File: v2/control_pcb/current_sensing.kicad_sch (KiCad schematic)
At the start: 20 parts, among them J14 Conn_02x02_Top_Bottom, J15 Conn_02x02_Top_Bottom, U10 TMCS1108A3UQDR, U11 TMCS1108A3UQDR, U6 TMCS1108A3UQDR, U7 TMCS1108A3UQDR, U8 ADS7828, U9 LM4040LP-4.1

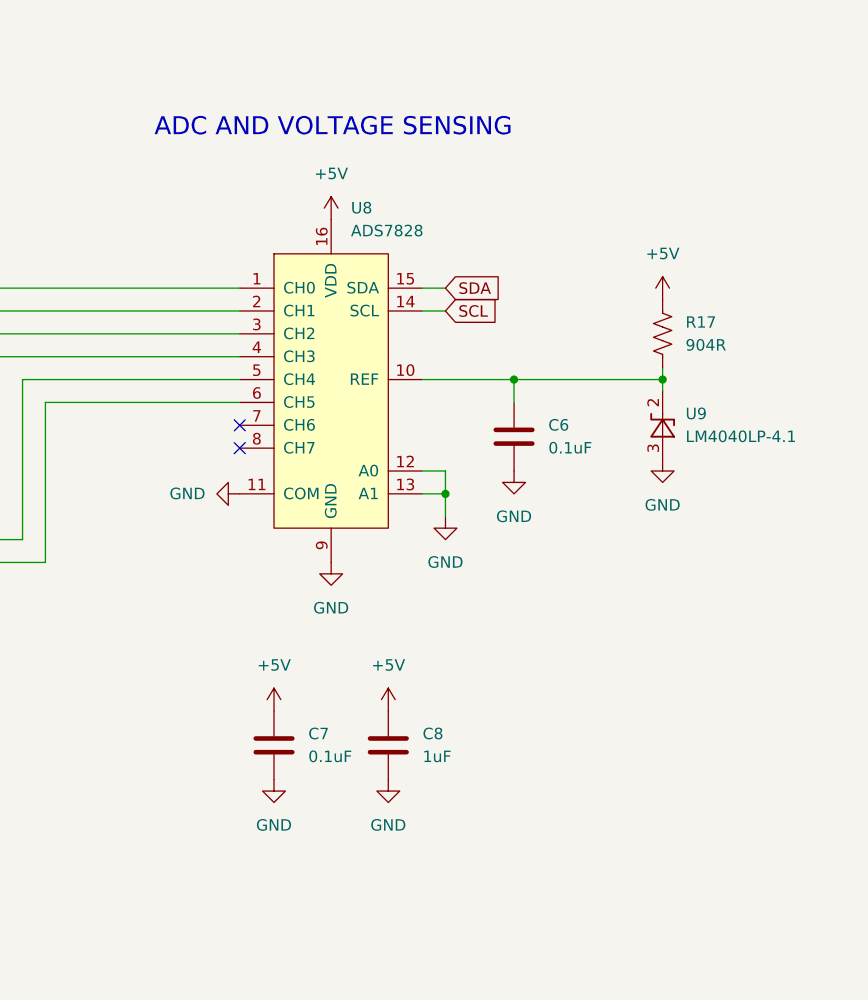
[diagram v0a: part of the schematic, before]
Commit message: Doing stuff
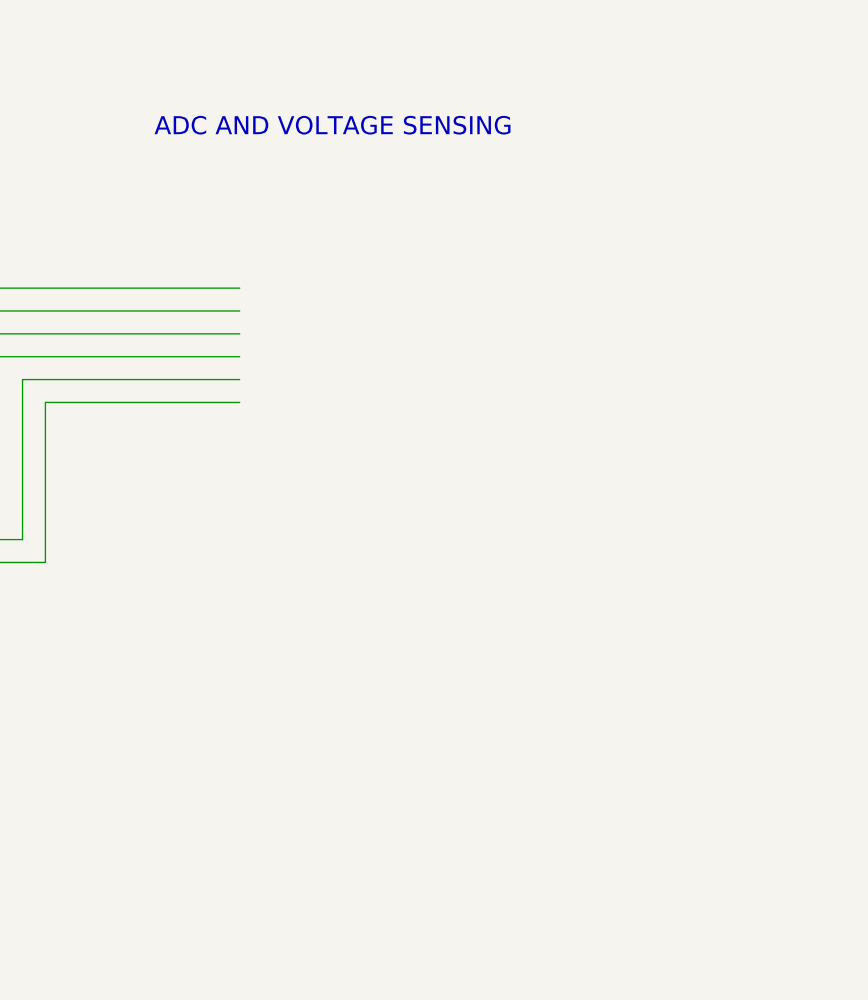
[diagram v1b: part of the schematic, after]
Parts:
- removed C6, C7: 0.1uF, Capacitor_THT:C_Rect_L4.6mm_W2.0mm_P2.50mm_MKS02_FKP02, symbol Device:C
- removed C8: 1uF, Capacitor_THT:C_Rect_L4.6mm_W2.0mm_P2.50mm_MKS02_FKP02, symbol Device:C
- removed R17: 904R, Resistor_THT:R_Axial_DIN0207_L6.3mm_D2.5mm_P10.16mm_Horizontal, symbol Device:R_US
- removed U8: ADS7828, Package_SO:TSSOP-16_4.4x5mm_P0.65mm, symbol Analog_ADC:ADS7828
- removed U9: LM4040LP-4.1, Package_TO_SOT_THT:TO-92_Inline, symbol Reference_Voltage:LM4040LP-4.1
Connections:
- no-connect marks 6 -> 4
